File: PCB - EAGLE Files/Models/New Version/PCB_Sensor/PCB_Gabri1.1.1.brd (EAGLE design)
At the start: 37 x 24 mm, 7 parts, among them U1 VEML6030, X1 0446200002

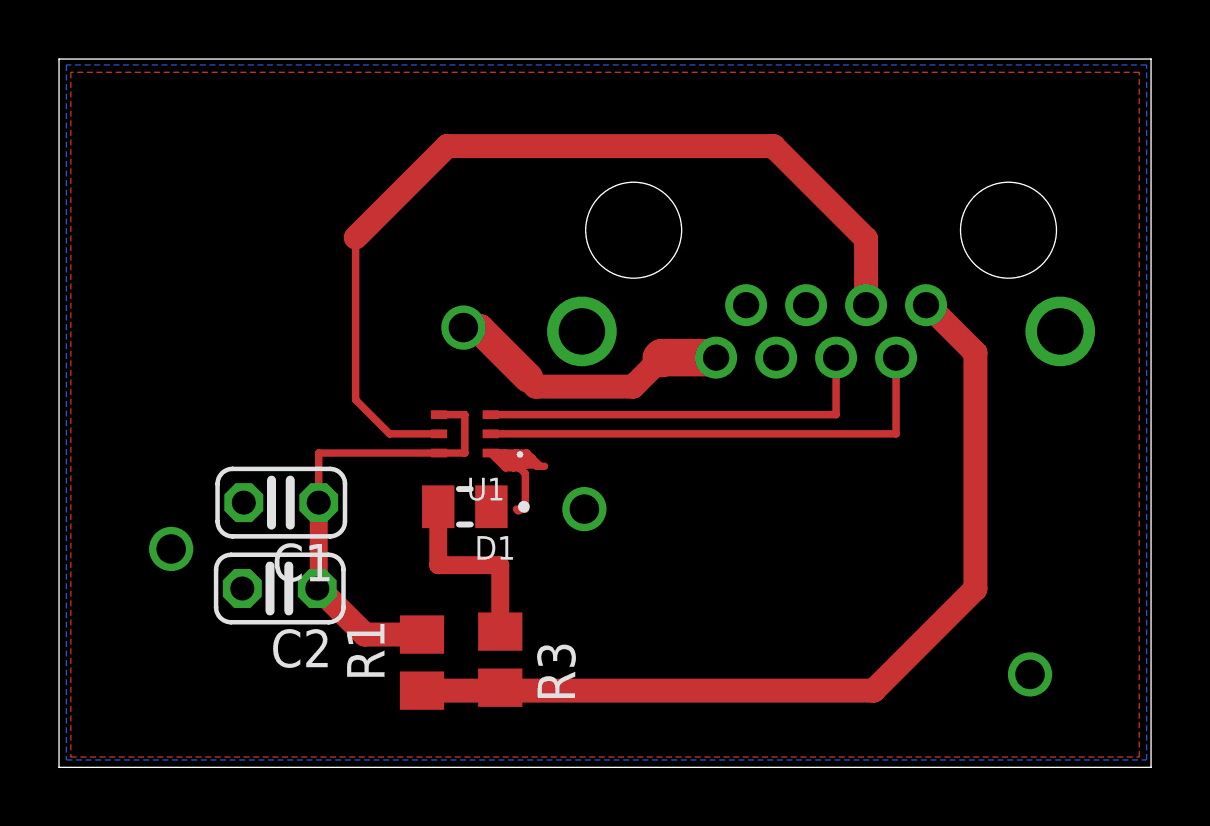
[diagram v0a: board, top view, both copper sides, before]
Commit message: Uploaded printings of final version pcb
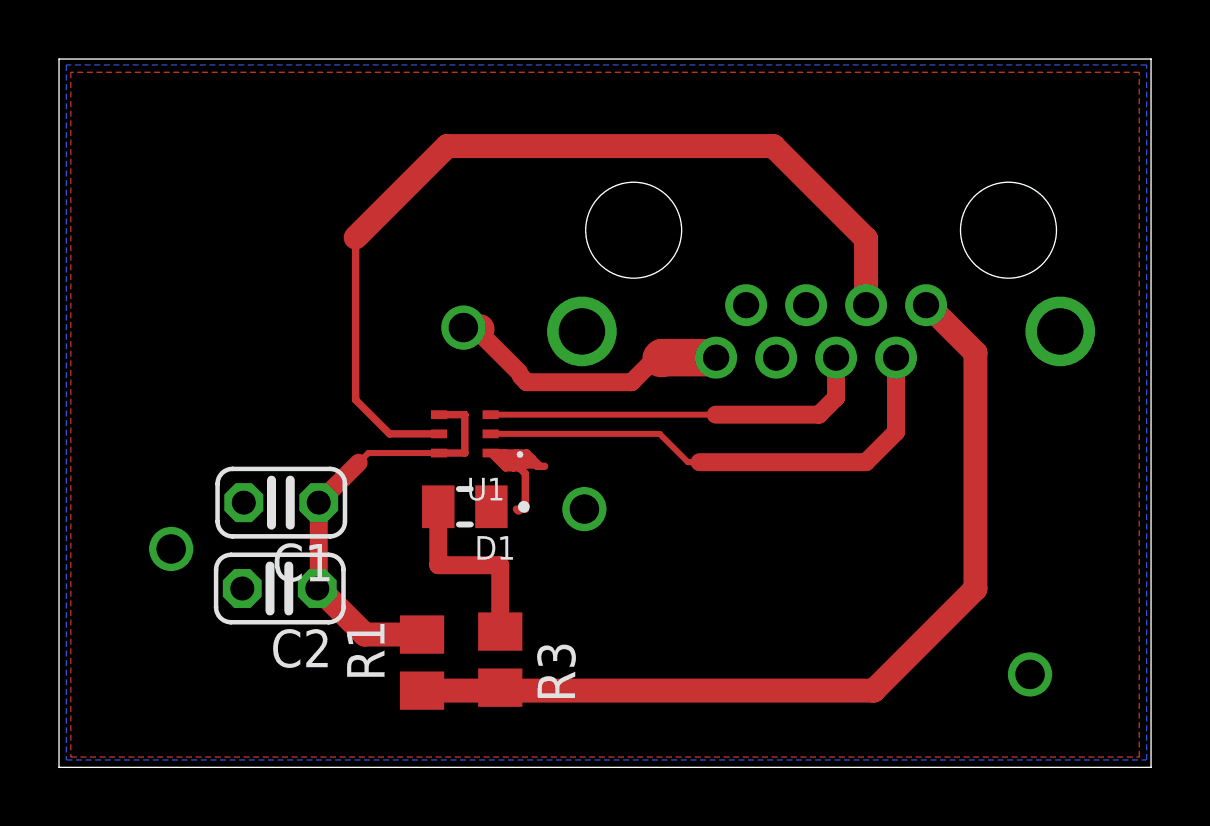
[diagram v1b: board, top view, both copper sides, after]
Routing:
- net LS_VDD: track 15.9 -> 14.8 mm
- net SDA: track 16.3 -> 17.1 mm
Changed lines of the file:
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@@
 <wire x1="66.8" y1="66.97" x2="66.8" y2="64.06" width="0.6096" layer="1"/>
 <wire x1="66.8" y1="64.06" x2="66.75" y2="64.06" width="0.6096" layer="1"/>
-<wire x1="70.875" y1="68.65" x2="66.8" y2="68.65" width="0.254" layer="1"/>
-<wire x1="66.8" y1="68.65" x2="66.8" y2="66.97" width="0.254" layer="1"/>
 <wire x1="70.875" y1="69.95" x2="71.75" y2="69.95" width="0.254" layer="1"/>
 <wire x1="71.75" y1="69.95" x2="71.75" y2="68.65" width="0.254" layer="1"/>
@@
 <wire x1="70.3" y1="62.5" x2="68.36" y2="62.5" width="0.8128" layer="1"/>
 <wire x1="68.36" y1="62.5" x2="66.8" y2="64.06" width="0.8128" layer="1"/>
+<wire x1="70.875" y1="68.65" x2="68.48" y2="68.65" width="0.2032" layer="1"/>
+<wire x1="68.48" y1="68.65" x2="68.265" y2="68.435" width="0.2032" layer="1"/>
+<wire x1="66.8" y1="66.97" x2="68.1525625" y2="68.3225625" width="0.6096" layer="1"/>
+<wire x1="68.1525625" y1="68.3225625" x2="68.265" y2="68.435" width="0" layer="19" extent="1-1"/>
 </signal>
 <signal name="3V3">
@@
 <contactref element="U1" pad="2"/>
 <contactref element="X1" pad="2"/>
-<wire x1="72.625" y1="69.3" x2="86.36" y2="69.3" width="0.254" layer="1"/>
-<wire x1="86.36" y1="69.3" x2="86.36" y2="71.882" width="0.254" layer="1"/>
+<wire x1="72.625" y1="69.3" x2="78.35" y2="69.3" width="0.2032" layer="1"/>
+<wire x1="86.36" y1="71.882" x2="86.36" y2="69.36" width="0.6096" layer="1"/>
+<wire x1="79.7" y1="68.3404" x2="85.3404" y2="68.3404" width="0.6096" layer="1"/>
+<wire x1="86.36" y1="69.36" x2="85.3404" y2="68.3404" width="0.6096" layer="1"/>
+<wire x1="79.3096" y1="68.3404" x2="79.7" y2="68.3404" width="0.2032" layer="1"/>
+<wire x1="78.35" y1="69.3" x2="79.3096" y2="68.3404" width="0.2032" layer="1"/>
 </signal>
 <signal name="INT">
 <contactref element="U1" pad="3"/>
 <contactref element="X1" pad="4"/>
-<wire x1="72.625" y1="69.95" x2="84.328" y2="69.95" width="0.254" layer="1"/>
-<wire x1="84.328" y1="69.95" x2="84.328" y2="71.882" width="0.254" layer="1"/>
+<wire x1="80.25" y1="69.95" x2="72.625" y2="69.95" width="0.2032" layer="1"/>
+<wire x1="84.328" y1="71.882" x2="84.328" y2="70.528" width="0.6096" layer="1"/>
+<wire x1="84.328" y1="70.528" x2="83.75" y2="69.95" width="0.6096" layer="1"/>
+<wire x1="83.75" y1="69.95" x2="80.25" y2="69.95" width="0.6096" layer="1"/>
 </signal>
 <signal name="N$1">
@@
 <wire x1="72.5" y1="72.9" x2="71.7" y2="72.9" width="0.254" layer="1"/>
 <wire x1="71.65" y1="72.85" x2="72.25" y2="72.85" width="1.016" layer="1"/>
-<wire x1="72.25" y1="72.85" x2="73.9" y2="71.2" width="1.016" layer="1"/>
-<wire x1="74" y1="71.05" x2="74.15" y2="70.9" width="0.8128" layer="1"/>
-<wire x1="74.15" y1="70.9" x2="77.45" y2="70.9" width="0.8128" layer="1"/>
-<wire x1="78.4" y1="71.85" x2="77.45" y2="70.9" width="0.8128" layer="1"/>
 <wire x1="80.264" y1="71.882" x2="78.432" y2="71.882" width="1.27" layer="1"/>
 <wire x1="78.432" y1="71.882" x2="78.4" y2="71.85" width="1.27" layer="1"/>
+<wire x1="71.7" y1="72.9" x2="72.07280625" y2="72.9" width="0.6096" layer="1"/>
+<wire x1="72.07280625" y1="72.9" x2="73.59100625" y2="71.3818" width="0.6096" layer="1"/>
+<wire x1="73.65" y1="71.25" x2="73.85" y2="71.05" width="0.6096" layer="1"/>
+<wire x1="73.85" y1="71.05" x2="77.4" y2="71.05" width="0.6096" layer="1"/>
+<wire x1="77.4" y1="71.05" x2="78.3" y2="71.95" width="0.6096" layer="1"/>
+<wire x1="78.3" y1="71.95" x2="78.35" y2="71.95" width="0.6096" layer="1"/>
+<wire x1="80.264" y1="71.882" x2="90.9" y2="61.15" width="0" layer="19" extent="1-1"/>
+<wire x1="78.35" y1="71.95" x2="78.432" y2="71.882" width="0" layer="19" extent="1-1"/>
+<wire x1="73.59100625" y1="71.3818" x2="73.65" y2="71.25" width="0" layer="19" extent="1-1"/>
+<wire x1="71.65" y1="72.85" x2="71.7" y2="72.9" width="0" layer="19" extent="1-1"/>
+<wire x1="73.85" y1="68.65" x2="73.85" y2="71.05" width="0" layer="19" extent="1-1"/>
+<wire x1="72.65" y1="66.83" x2="73.5" y2="66.75" width="0" layer="19" extent="1-1"/>
+<wire x1="75.8" y1="66.75" x2="74.45" y2="68.2" width="0" layer="19" extent="1-1"/>
+<wire x1="64.26" y1="66.97" x2="72.65" y2="66.83" width="0" layer="19" extent="1-1"/>
+<wire x1="64.21" y1="64.06" x2="64.26" y2="66.97" width="0" layer="19" extent="1-1"/>
+<wire x1="61.8" y1="65.4" x2="64.21" y2="64.06" width="0" layer="19" extent="1-1"/>
 </signal>
 </signals>
